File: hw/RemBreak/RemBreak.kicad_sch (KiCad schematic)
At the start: 6 parts, among them J2 Conn_02x06_Odd_Even

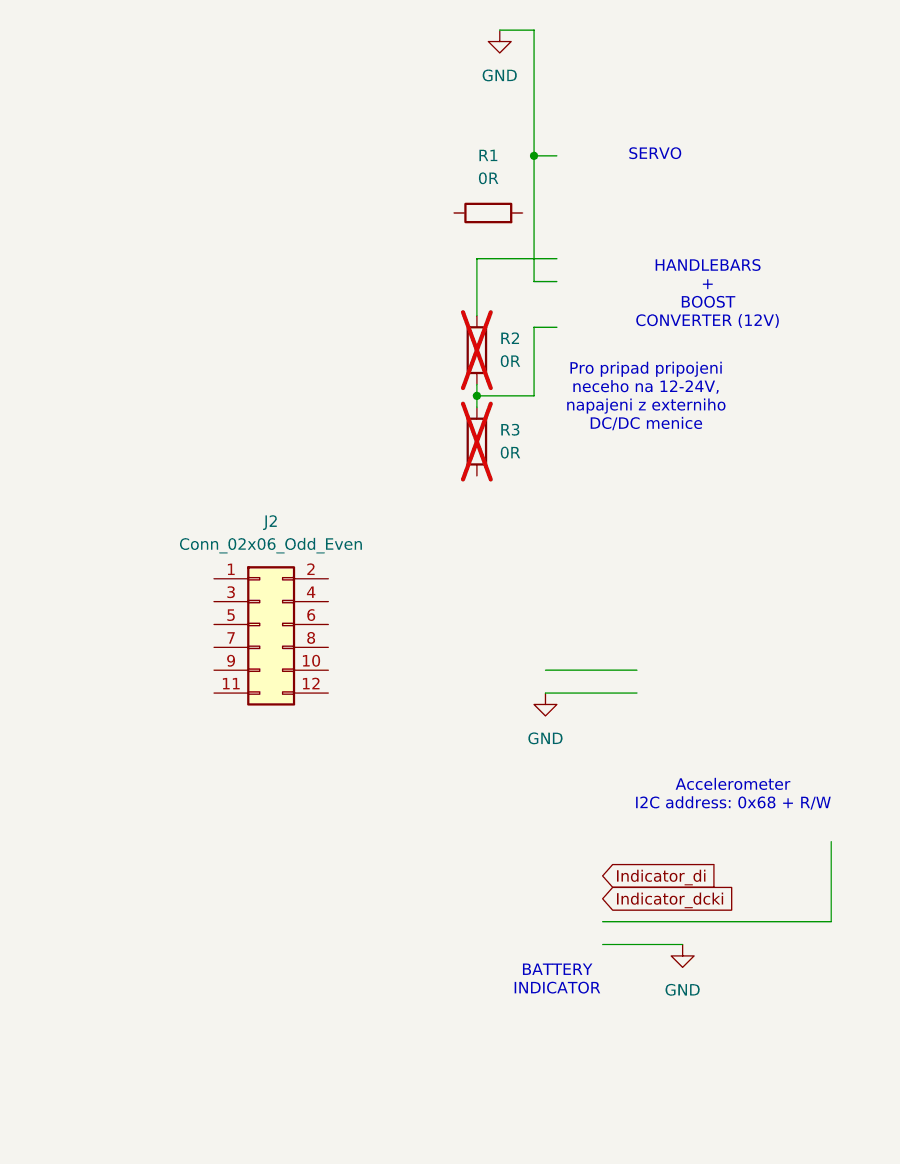
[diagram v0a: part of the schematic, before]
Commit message: updated pcb and schematics - still in progress
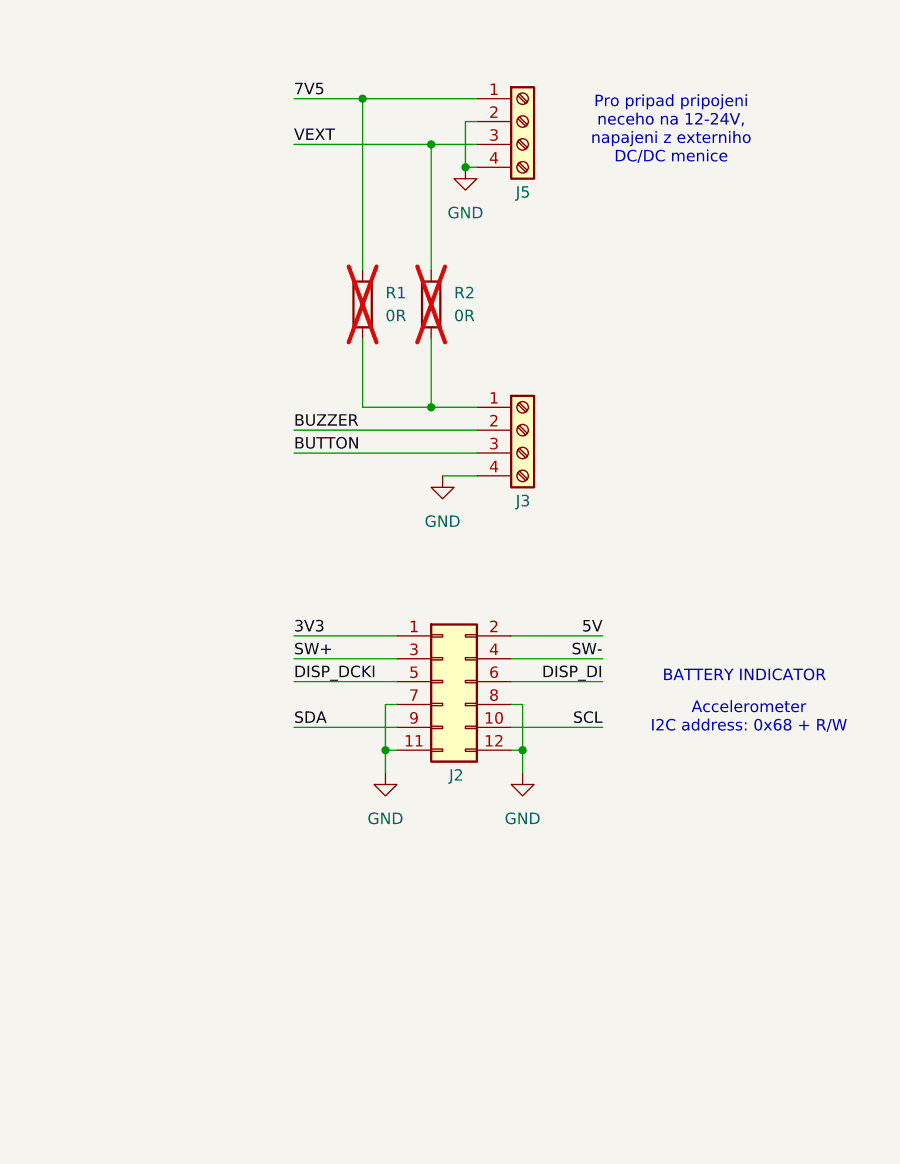
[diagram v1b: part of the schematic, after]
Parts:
- removed R3: 0R, Resistor_SMD:R_0805_2012Metric, symbol Device:R
- added J3, J5: Screw_Terminal_01x04, TerminalBlock_Phoenix:TerminalBlock_Phoenix_MPT-0,5-4-2.54_1x04_P2.54mm_Horizontal, symbol Connector:Screw_Terminal_01x04
- J2: footprint Connector_PinHeader_2.54mm:PinHeader_2x06_P2.54mm_Vertical_SMD -> dodo_conn:SAMTEC_TSM-106-01-L-DH-P-TR
- R1: now not fitted
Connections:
- net GND: now also J2.11 (Pin_11), J2.12 (Pin_12), J2.7 (Pin_7), J2.8 (Pin_8), J3.4 (Pin_4), J5.2 (Pin_2), J5.4 (Pin_4)
- net 7V5: now reaches R1.1
- net 7V5: now also J5.1 (Pin_1)
- net at R1.2: now also R2.2, J3.1 (Pin_1)
- net VEXT: now reaches R2.1
- net VEXT: now also J5.3 (Pin_3)
- net 3V3: now reaches J2.1 (Pin_1)
- net SCL: now reaches J2.10 (Pin_10)
- net 5V: now reaches J2.2 (Pin_2)
- net SW+: now reaches J2.3 (Pin_3)
- net SW-: now reaches J2.4 (Pin_4)
- net DISP_DCKI: now reaches J2.5 (Pin_5)
- net DISP_DI: now reaches J2.6 (Pin_6)
- net SDA: now reaches J2.9 (Pin_9)
- new net BUTTON: J3.3 (Pin_3)
- new net BUZZER: J3.2 (Pin_2)
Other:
- note removed: "HANDLEBARS + BOOST CONVERTER (12V)"
- note removed: "SERVO"
- moved on the sheet: J2
